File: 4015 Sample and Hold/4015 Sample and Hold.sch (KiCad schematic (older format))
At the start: 46 parts, among them J1 INPUT, J4 SAMPLE IN, J5 OUTPUT, J6 POSITIVE SUPPLY, J7 GROUND, J8 NEGATIVE SUPPLY, Q1 2N5172, Q2 2N3906, Q3 2N5172, Q4 BF245A or 2SK30, Q5 2N3906, Q6 2N5172, Q7-1 BF245A or 2SK30, Q7-2 BF245A or 2SK30

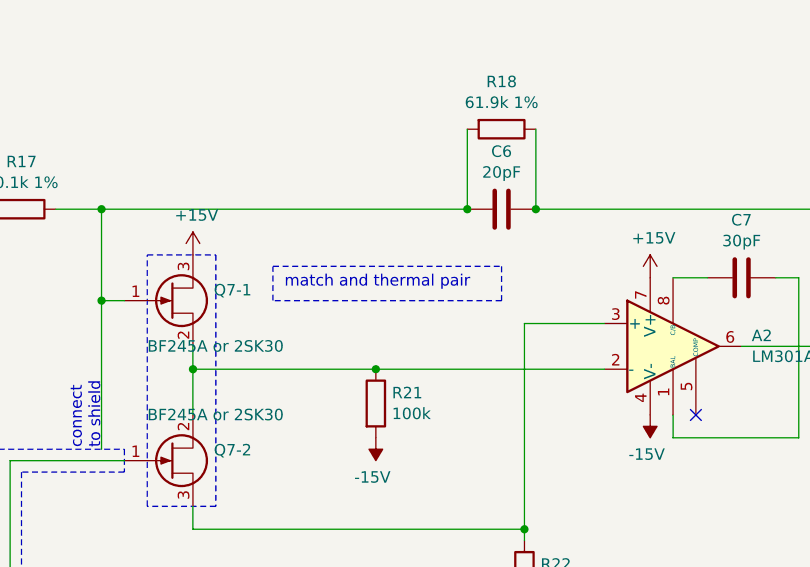
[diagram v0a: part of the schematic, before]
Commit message: various fixes
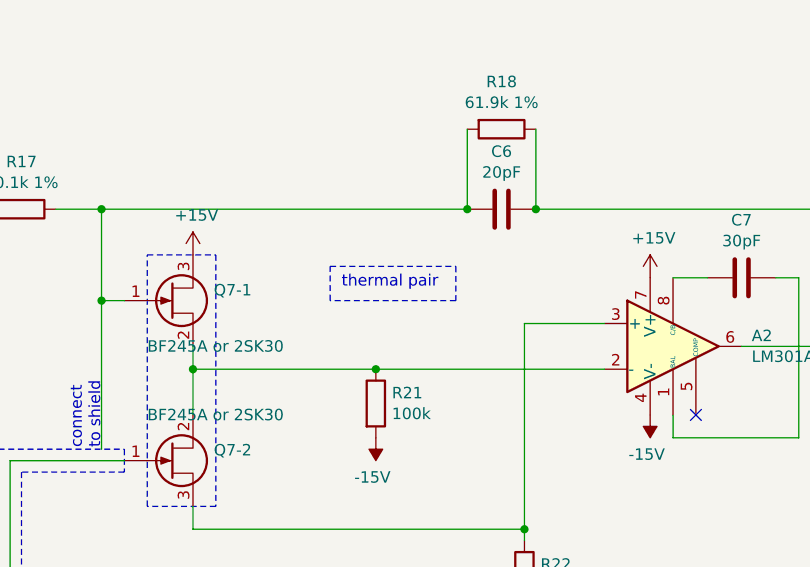
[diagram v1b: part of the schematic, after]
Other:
- note added: "thermal pair"
- note removed: "match and thermal pair"
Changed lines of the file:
@@
 Wire Wire Line
 	8400 3400 8400 2500
-Text Notes 7350 2350 0    50   ~ 0
-match and thermal pair
+Text Notes 7600 2350 0    50   ~ 0
+thermal pair
 Wire Notes Line
-	7300 2250 8300 2250
+	7550 2250 8100 2250
 Wire Notes Line
-	8300 2250 8300 2400
+	8100 2250 8100 2400
 Wire Notes Line
-	8300 2400 7300 2400
+	8100 2400 7550 2400
 Wire Notes Line
-	7300 2400 7300 2250
+	7550 2400 7550 2250
 $EndSCHEMATC
